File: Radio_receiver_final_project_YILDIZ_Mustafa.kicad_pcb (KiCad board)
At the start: 2 copper layers, 90.5 x 27.1 mm, 26 parts, among them T1 BF199, T2 BC547, T3 BC547, T4 BC547

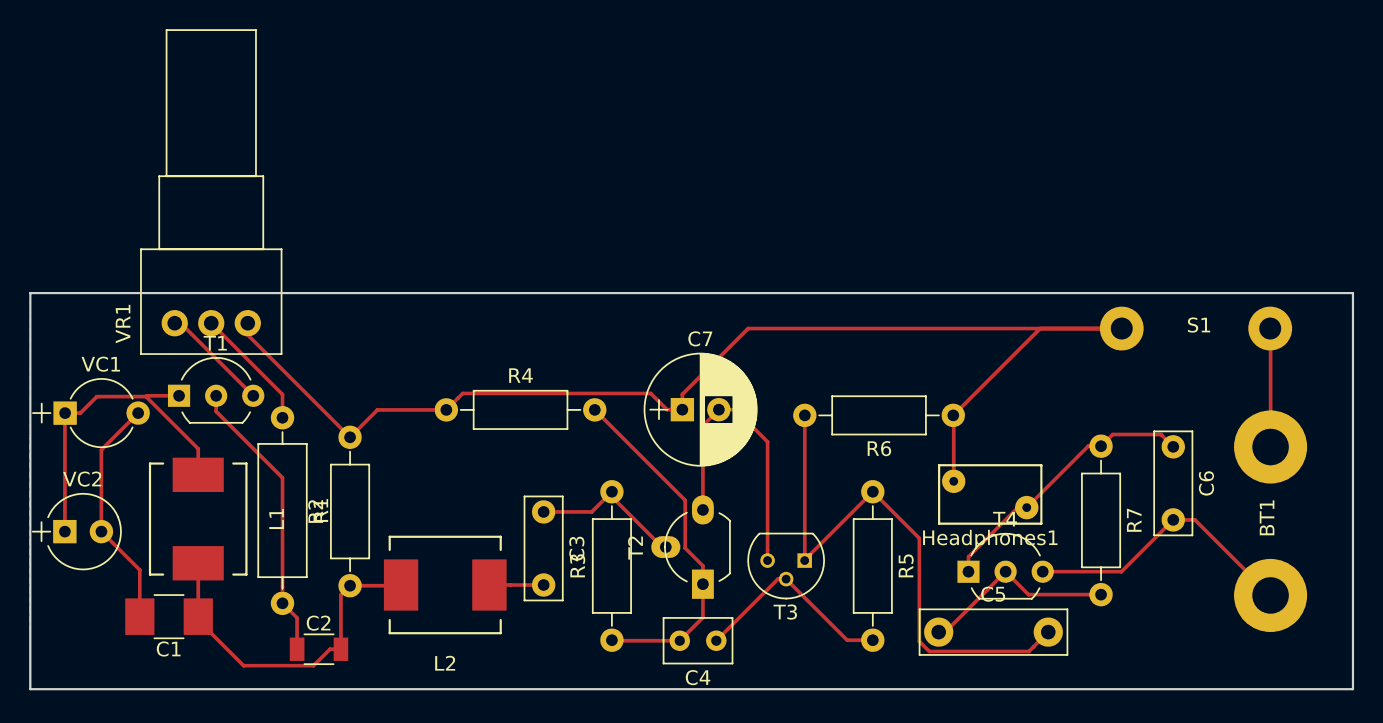
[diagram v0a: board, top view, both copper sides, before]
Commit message: some shanges
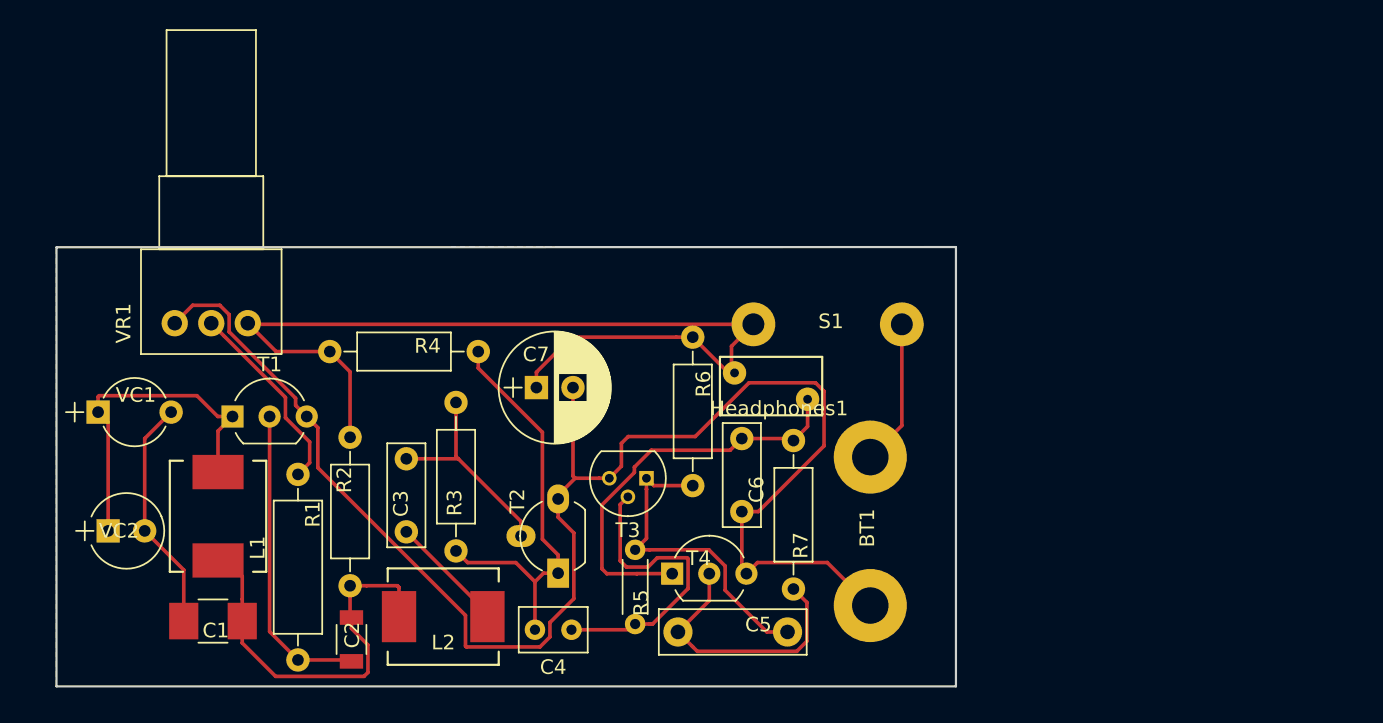
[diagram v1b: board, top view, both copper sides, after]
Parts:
- R5: footprint Resistors_THT:R_Axial_DIN0207_L6.3mm_D2.5mm_P10.16mm_Horizontal -> Resistors_THT:R_Axial_DIN0204_L3.6mm_D1.6mm_P5.08mm_Horizontal
- moved C6 29.5 mm to (127.5, 102.4)
- moved BT1 27.4 mm to (136.3, 103.6)
- moved S1 25.2 mm to (138.4, 94.6)
- moved R7 21.1 mm to (131.0, 102.5)
- moved T4 20.3 mm to (122.7, 111.6)
- moved R6 18.6 mm to (124.1, 95.4), turned to 270 degrees
- moved C5 17.8 mm to (123.1, 115.6)
- moved R5 16.7 mm to (120.2, 110.0)
- moved Headphones1 16.7 mm to (127.0, 97.9)
- moved R3 12.3 mm to (107.9, 110.1)
- moved T3 12.2 mm to (121.0, 105.1)
- moved C7 10.1 mm to (113.4, 98.9)
- moved C3 10.1 mm to (104.5, 103.8)
- moved C4 9.94 mm to (115.8, 115.5)
- moved T2 9.94 mm to (114.9, 111.6)
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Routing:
- net Net-(BT1-Pad2): track 46.3 -> 105.2 mm
- net Net-(C7-Pad1): track 86.7 -> 68.1 mm
- net Net-(C5-Pad2): track 37.8 -> 22.3 mm
- net Net-(C6-Pad1): track 19.0 -> 27.8 mm
- net Net-(C4-Pad1): track 14.2 -> 20.9 mm
- net Net-(C5-Pad1): track 13.5 -> 18.5 mm
- net Net-(R1-Pad1): track 8.49 -> 13.5 mm
- net Net-(C4-Pad2): track 24.2 -> 28.8 mm
- net Net-(C1-Pad1): track 23.5 -> 28.2 mm
- net Net-(C3-Pad2): track 3.71 -> 8.10 mm
- net Net-(C3-Pad1): track 10.7 -> 14.5 mm
- net Net-(BT1-Pad1): track 8.12 -> 9.98 mm
- net Net-(C2-Pad1): track 19.6 -> 21.2 mm
- added copper zone on B.Cu, net Net-(BT1-Pad2)
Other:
- board size 90.5 x 27.1 mm -> 61.6 x 30.1 mm
